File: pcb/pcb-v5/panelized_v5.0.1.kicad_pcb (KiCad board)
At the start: 2 copper layers, 99.6 x 99.8 mm, 55 parts, among them J1 Conn_01x05_Female, J2 Conn_01x05_Female, J3 Conn_01x05_Female, J4 Conn_01x05_Male, Q1 2N7002, SW1 G71Y, SW2 G71Y, SW3 G71Y, U1 AMS1117-3.3

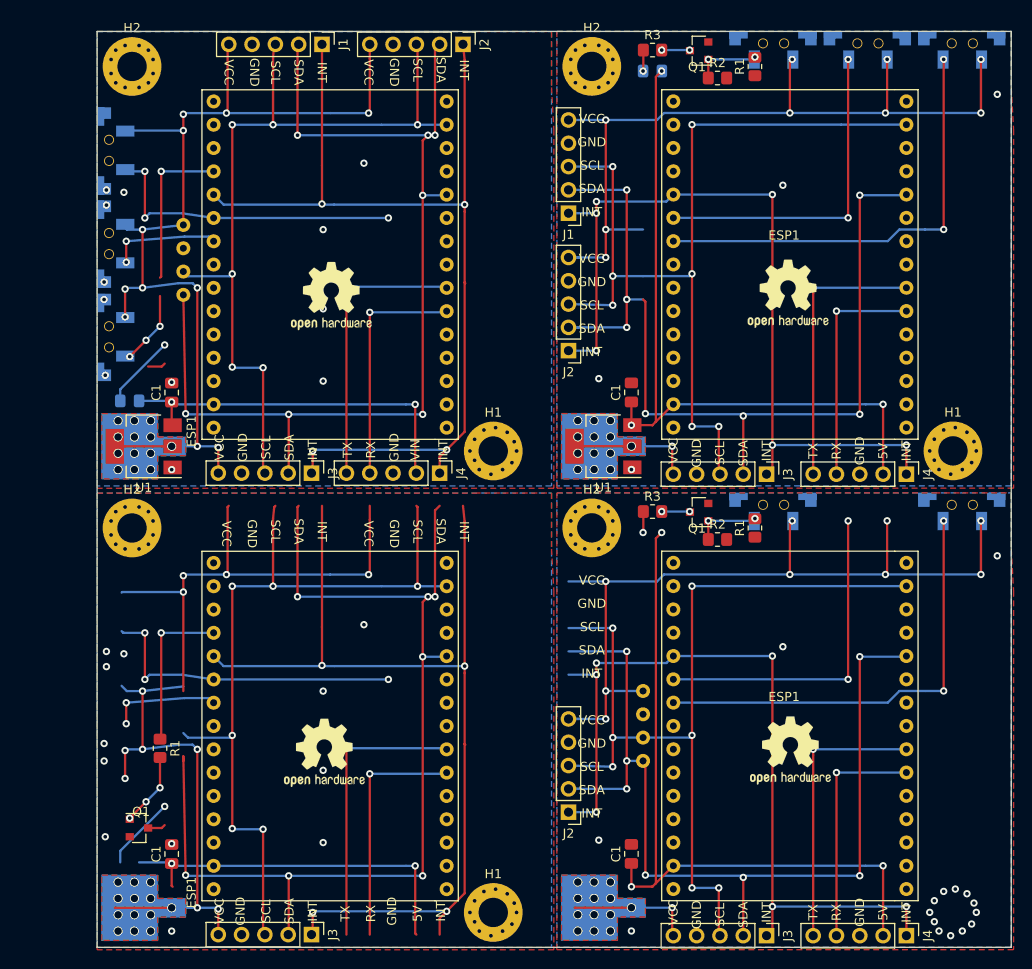
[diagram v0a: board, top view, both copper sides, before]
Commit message: PCB-V5 update
Panelized version 1.0.0
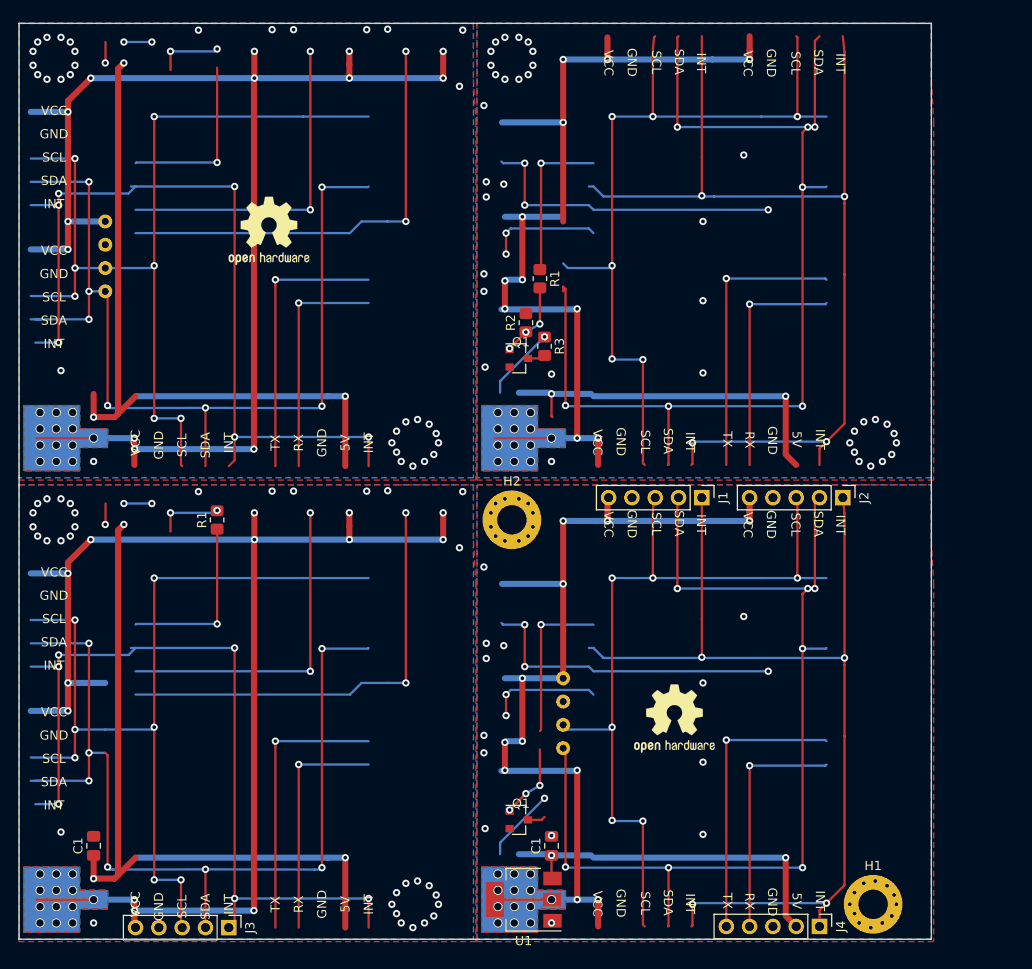
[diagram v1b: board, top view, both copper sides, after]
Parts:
- removed the C1 at (136.1, 121.1)
- removed the C1 at (86.0, 121.1)
- removed the C1 at (86.0, 70.8)
- removed the C1 at (136.1, 70.8)
- removed D1 (x2): LED, LED_SMD:LED_0805_2012Metric_Pad1.15x1.40mm_HandSolder
- removed ESP1 (x4): ESP32, pcb-v5:ESP32_30_pins
- removed the H1 at (121.0, 127.5)
- removed the H1 at (121.0, 77.2)
- removed the H1 at (171.1, 77.2)
- removed the H2 at (131.8, 85.6)
- removed the H2 at (81.7, 85.6)
- removed the H2 at (81.7, 35.3)
- removed the H2 at (131.8, 35.3)
- removed the J1 at (102.4, 32.9)
- removed the J1 at (129.2, 51.3)
- removed the J2 at (129.2, 116.6)
- removed the J2 at (117.7, 32.9)
- removed the J2 at (129.2, 66.3)
- removed the J3 at (150.8, 130.0)
- removed the J3 at (101.2, 129.9)
- removed the J3 at (101.2, 79.6)
- removed the J3 at (150.8, 79.7)
- removed the J4 at (166.1, 130.0)
- removed the J4 at (115.2, 79.6)
- removed the J4 at (166.1, 79.7)
- removed the OLED1 at (169.1, 89.4)
- removed the OLED1 at (119.0, 38.6)
- removed the Q1 at (143.5, 83.9)
- removed the Q1 at (82.4, 118.3)
- removed the Q1 at (143.5, 33.6)
- removed the R1 at (149.6, 85.6)
- removed the R1 at (84.7, 109.6)
- removed the R1 at (149.6, 35.3)
- removed the R2 at (145.5, 86.9)
- removed the R2 at (145.5, 36.6)
- removed the R3 at (138.4, 83.8)
- removed the R3 at (138.4, 33.5)
- removed the REF** at (153.4, 109.9)
- removed the REF** at (102.6, 110.1)
- removed the REF** at (153.2, 60.1)
- removed the REF** at (103.4, 60.3)
- removed SW1 (x3), SW2 (x2), SW3 (x3): G71Y, pcb-v5:G71Y_µsw_smd
- removed the U1 at (82.9, 76.7)
- removed the U1 at (133.0, 76.7)
- added C1: 10µF, Capacitor_SMD:C_0805_2012Metric_Pad1.18x1.45mm_HandSolder, F.Cu at (127.4, 120.3)
- added C1: 10µF, Capacitor_SMD:C_0805_2012Metric_Pad1.18x1.45mm_HandSolder, F.Cu at (77.5, 120.3)
- added H1: MountingHole_Pad, MountingHole:MountingHole_3.2mm_M3_Pad, F.Cu at (162.4, 126.6)
- added H2: MountingHole_Pad, MountingHole:MountingHole_3.2mm_M3_Pad, F.Cu at (123.1, 84.7)
- added J1: Conn_01x05_Female, Connector_PinHeader_2.54mm:PinHeader_1x05_P2.54mm_Vertical, F.Cu at (143.8, 82.3)
- added J2: Conn_01x05_Female, Connector_PinHeader_2.54mm:PinHeader_1x05_P2.54mm_Vertical, F.Cu at (159.1, 82.3)
- added J3: Conn_01x05_Female, Connector_PinHeader_2.54mm:PinHeader_1x05_P2.54mm_Vertical, F.Cu at (92.2, 129.2)
- added J4: Conn_01x05_Male, Connector_PinHeader_2.54mm:PinHeader_1x05_P2.54mm_Vertical, F.Cu at (156.6, 129.0)
- added OLED1: OLED_1.3, pcb-v5:OLED_1.3, B.Cu at (160.4, 88.0)
- added OLED1: OLED_1.3, pcb-v5:OLED_1.3, B.Cu at (110.5, 38.2)
- added Q1: 2N7002, Package_TO_SOT_SMD:SOT-23, F.Cu at (123.8, 117.4)
- added Q1: 2N7002, Package_TO_SOT_SMD:SOT-23, F.Cu at (123.8, 67.1)
- added R1: 470, Resistor_SMD:R_0805_2012Metric_Pad1.20x1.40mm_HandSolder, F.Cu at (90.9, 84.7)
- added R1: 470, Resistor_SMD:R_0805_2012Metric_Pad1.20x1.40mm_HandSolder, F.Cu at (126.1, 58.4)
- added R2: 15k, Resistor_SMD:R_0805_2012Metric_Pad1.20x1.40mm_HandSolder, F.Cu at (124.6, 63.2)
- added R3: 68, Resistor_SMD:R_0805_2012Metric_Pad1.20x1.40mm_HandSolder, F.Cu at (126.6, 65.8)
- added REF**: OSHW-Logo2_9.8x8mm_SilkScreen, Symbol:OSHW-Logo2_9.8x8mm_SilkScreen, F.Cu at (140.8, 106.4)
- added REF**: OSHW-Logo2_9.8x8mm_SilkScreen, Symbol:OSHW-Logo2_9.8x8mm_SilkScreen, F.Cu at (96.6, 53.2)
- added U1: AMS1117-3.3, Package_TO_SOT_SMD:SOT-223-3_TabPin2, F.Cu at (124.3, 126.1)
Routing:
- net 3V3: track 422.7 -> 502.9 mm, vias 94 -> 100
- net GPIO_34: track 34.7 -> 73.2 mm, vias 2 -> 4
- net GPIO_32: track 141.6 -> 140.5 mm
- net VIN: track 234.7 -> 233.8 mm
- net SDA: track 431.0 -> 431.6 mm
- net GND: vias 128 -> 140
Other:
- board size 99.6 x 99.8 mm -> 99.4 x 99.8 mm
- board text removed: "VIN"
